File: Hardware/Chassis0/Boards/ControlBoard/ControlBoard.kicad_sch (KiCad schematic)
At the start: 18 parts, among them J1 TBP02R2W-381-06BE, J11 Conn_02x10_Counter_Clockwise, J12 Conn_02x10_Counter_Clockwise, J13 Conn_02x10_Counter_Clockwise, J14 Conn_02x10_Counter_Clockwise, J2 TBP02R2W-381-06BE, J3 TBP01R2W-508-02BE, J4 TBP01R1-508-04BE, J5 Conn_02x10_Counter_Clockwise, J7 TBP02R2W-381-08BE, J8 TBP02R2W-381-08BE

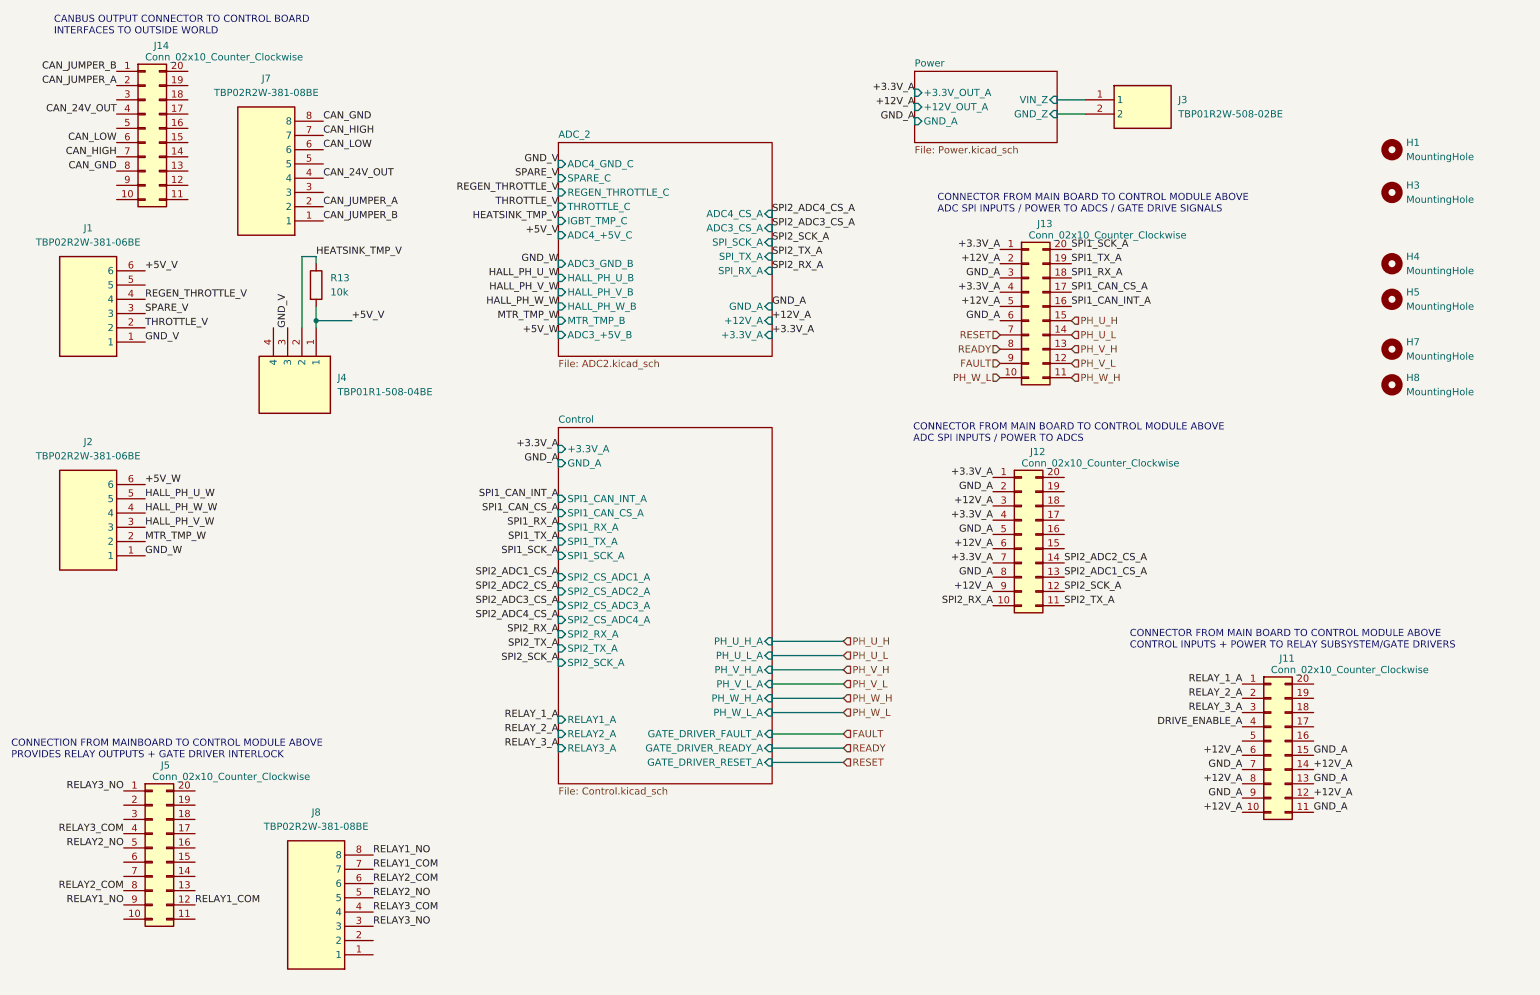
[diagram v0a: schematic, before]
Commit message: Update size 0 cad model
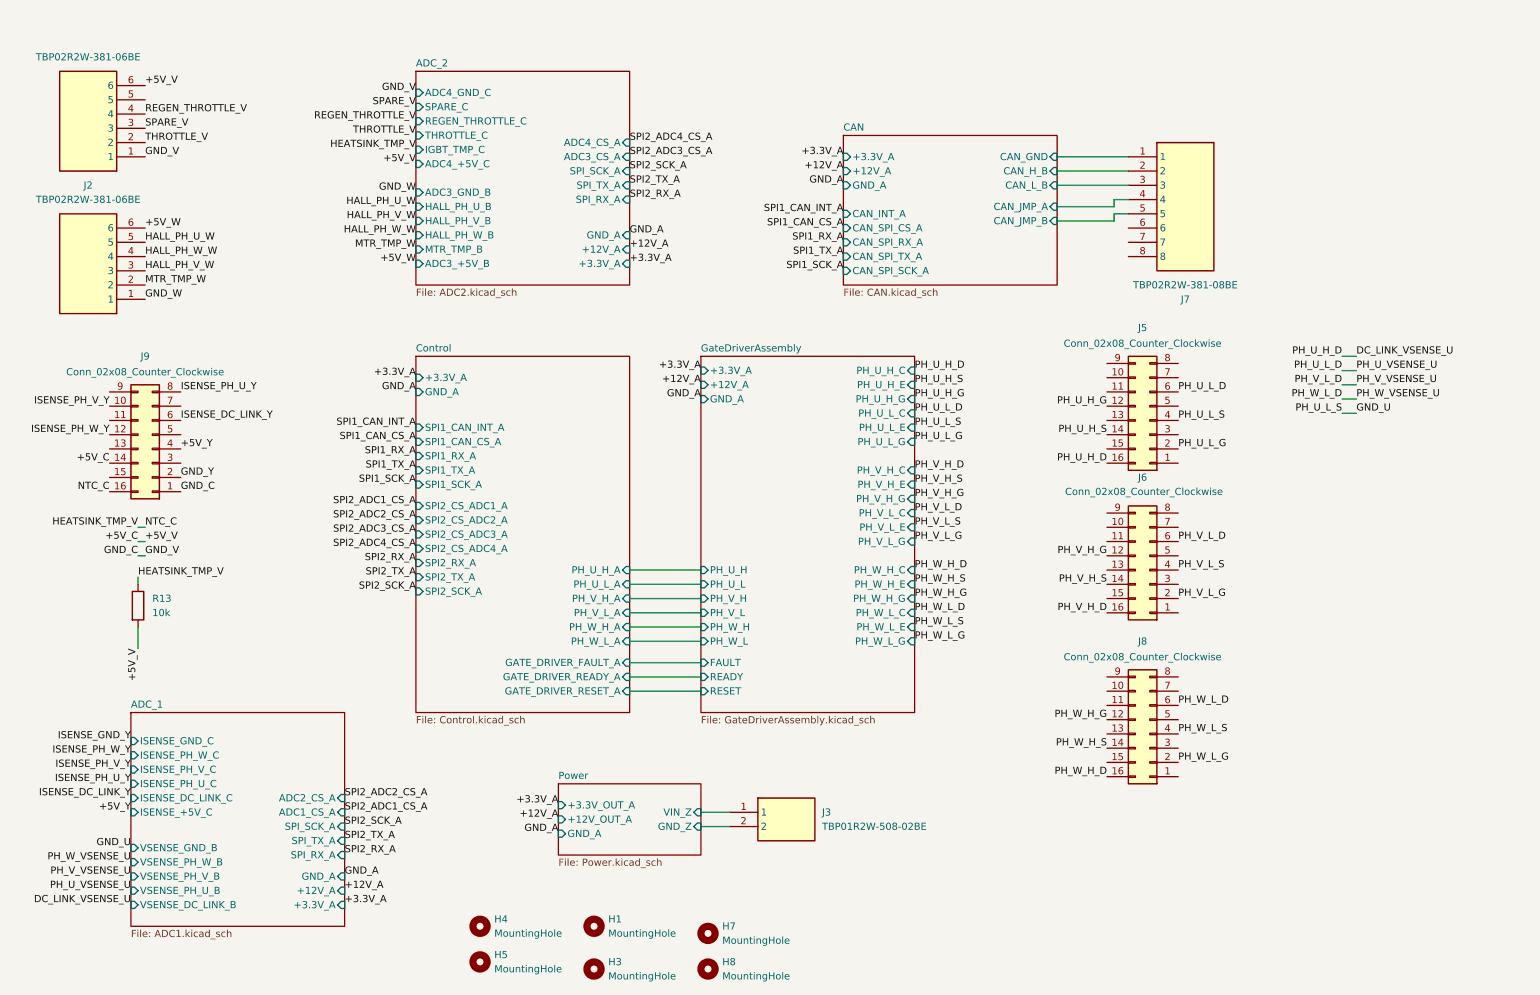
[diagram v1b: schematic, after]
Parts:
- removed J11, J12, J13, J14, J5: Conn_02x10_Counter_Clockwise, Connector_PinSocket_2.54mm:PinSocket_2x10_P2.54mm_Vertical, symbol Connector_Generic:Conn_02x10_Counter_Clockwise
- removed J4: TBP01R1-508-04BE, InverterCom:TBP01R150804BE, symbol InverterCom:TBP01R1-508-04BE
- removed J8: TBP02R2W-381-08BE, InverterCom:TBP02R2W38108BE, symbol InverterCom:TBP02R2W-381-08BE
- added J5, J6, J8, J9: Conn_02x08_Counter_Clockwise, Connector_PinSocket_2.54mm:PinSocket_2x08_P2.54mm_Vertical, symbol Connector_Generic:Conn_02x08_Counter_Clockwise
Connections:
- net HEATSINK_TMP_V: now also J9.16 (Pin_16)
- net CAN/CAN_L_B: now reaches J7.3
- net CAN/CAN_JMP_B: now reaches J7.5
- net +5V_V renamed +5V_C
- net +5V_C: now also J9.14 (Pin_14)
- net CAN_24V_OUT renamed CAN/CAN_JMP_A
- net CAN_GND: no longer names the net of J7.8
- net CAN_HIGH: no longer names the net of J7.7
- net CAN_JUMPER_A renamed CAN/CAN_H_B
- net CAN_JUMPER_B renamed CAN/CAN_GND
- net CAN_LOW: no longer names the net of J7.6
- net GND_V renamed GND_C
- net GND_C: now also J9.1 (Pin_1)
- new net +5V_Y: J9.4 (Pin_4)
- new net DC_LINK_VSENSE_U: J5.16 (Pin_16)
- new net GND_U: J5.4 (Pin_4)
- new net GND_Y: J9.2 (Pin_2)
- new net ISENSE_DC_LINK_Y: J9.6 (Pin_6)
- new net ISENSE_PH_U_Y: J9.8 (Pin_8)
- new net ISENSE_PH_V_Y: J9.10 (Pin_10)
- new net ISENSE_PH_W_Y: J9.12 (Pin_12)
- new net PH_U_H_G: J5.12 (Pin_12)
- new net PH_U_H_S: J5.14 (Pin_14)
- new net PH_U_L_D: J5.6 (Pin_6)
- new net PH_U_L_G: J5.2 (Pin_2)
- new net PH_V_H_D: J6.16 (Pin_16)
- new net PH_V_H_G: J6.12 (Pin_12)
- new net PH_V_H_S: J6.14 (Pin_14)
- new net PH_V_L_D: J6.6 (Pin_6)
- new net PH_V_L_G: J6.2 (Pin_2)
- new net PH_V_L_S: J6.4 (Pin_4)
- new net PH_W_H_D: J8.16 (Pin_16)
- new net PH_W_H_G: J8.12 (Pin_12)
- new net PH_W_H_S: J8.14 (Pin_14)
- new net PH_W_L_D: J8.6 (Pin_6)
- new net PH_W_L_G: J8.2 (Pin_2)
- new net PH_W_L_S: J8.4 (Pin_4)
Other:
- added sheet ADC_1 (ADC1.kicad_sch)
- added sheet CAN (CAN.kicad_sch)
- added sheet GateDriverAssembly (GateDriverAssembly.kicad_sch)
- sheet Control ports: added none; removed RELAY1_A, RELAY2_A, RELAY3_A
- note removed: "CANBUS OUTPUT CONNECTOR TO CONTROL BOARD INTERFACES TO OUTSIDE WORLD"
- note removed: "CONNECTION FROM MAINBOARD TO CONTROL MODULE ABOVE PROVIDES RELAY OUTPUTS + GATE DRIVER INTERLOCK"
- note removed: "CONNECTOR FROM MAIN BOARD TO CONTROL MODULE ABOVE ADC SPI INPUTS / POWER TO ADCS"
- note removed: "CONNECTOR FROM MAIN BOARD TO CONTROL MODULE ABOVE ADC SPI INPUTS / POWER TO ADCS / GATE DRIVE SIGNALS"
- note removed: "CONNECTOR FROM MAIN BOARD TO CONTROL MODULE ABOVE CONTROL INPUTS + POWER TO RELAY SUBSYSTEM/GATE DRIVERS"
- moved on the sheet: H1, H3, H4, H5, H7, H8, J2, J3, J7, R13
